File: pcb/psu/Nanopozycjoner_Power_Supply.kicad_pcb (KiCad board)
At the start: 2 copper layers, 73 x 80 mm, 132 parts, among them J1 Conn_01x02_Socket, J2 Conn_01x02_Socket, J3 Conn_01x02_Socket, J4 Conn_01x02_Socket, J5 Conn_01x02_Socket, J6 Conn_01x02_Socket, J7 Conn_01x02_Socket, J8 Conn_01x02_Socket, U1 ADPL16000B, U2 LTC3260xDE, U3 ADPL54203, U4 ADPL54203

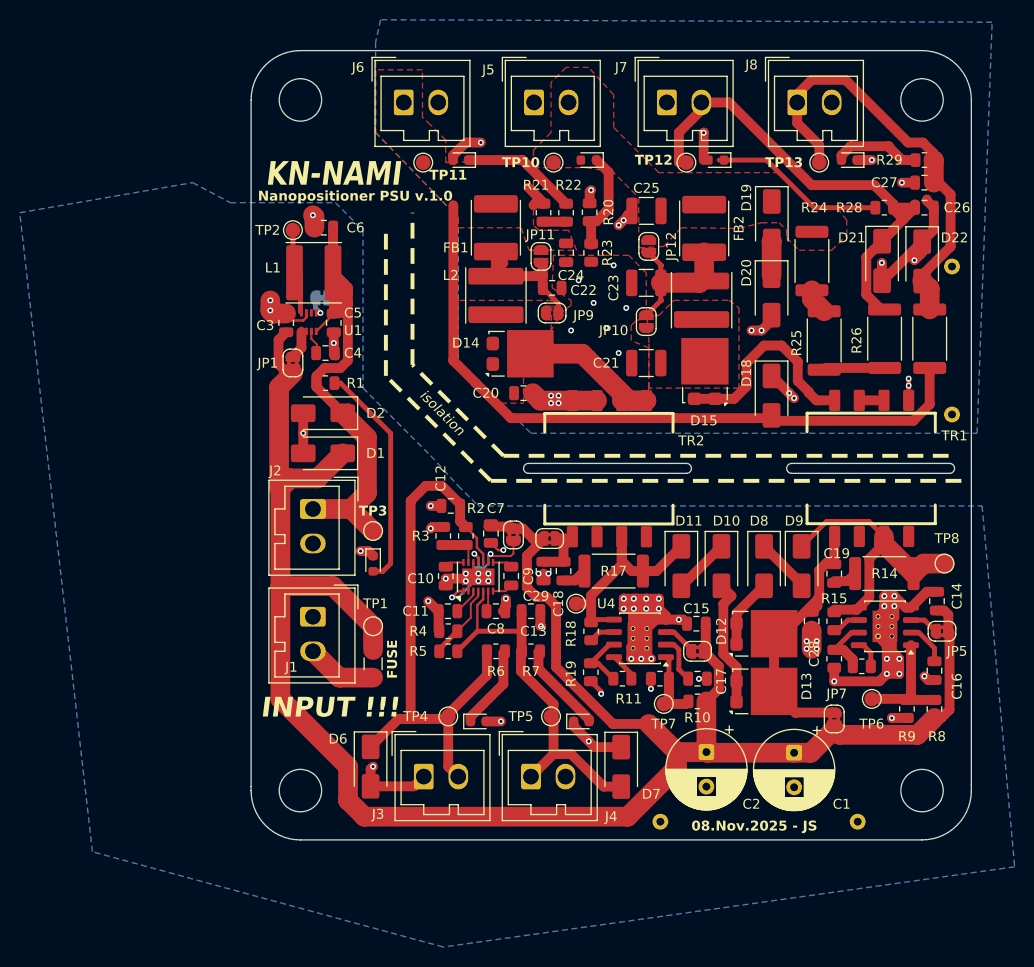
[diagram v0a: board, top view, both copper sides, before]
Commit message: final changes
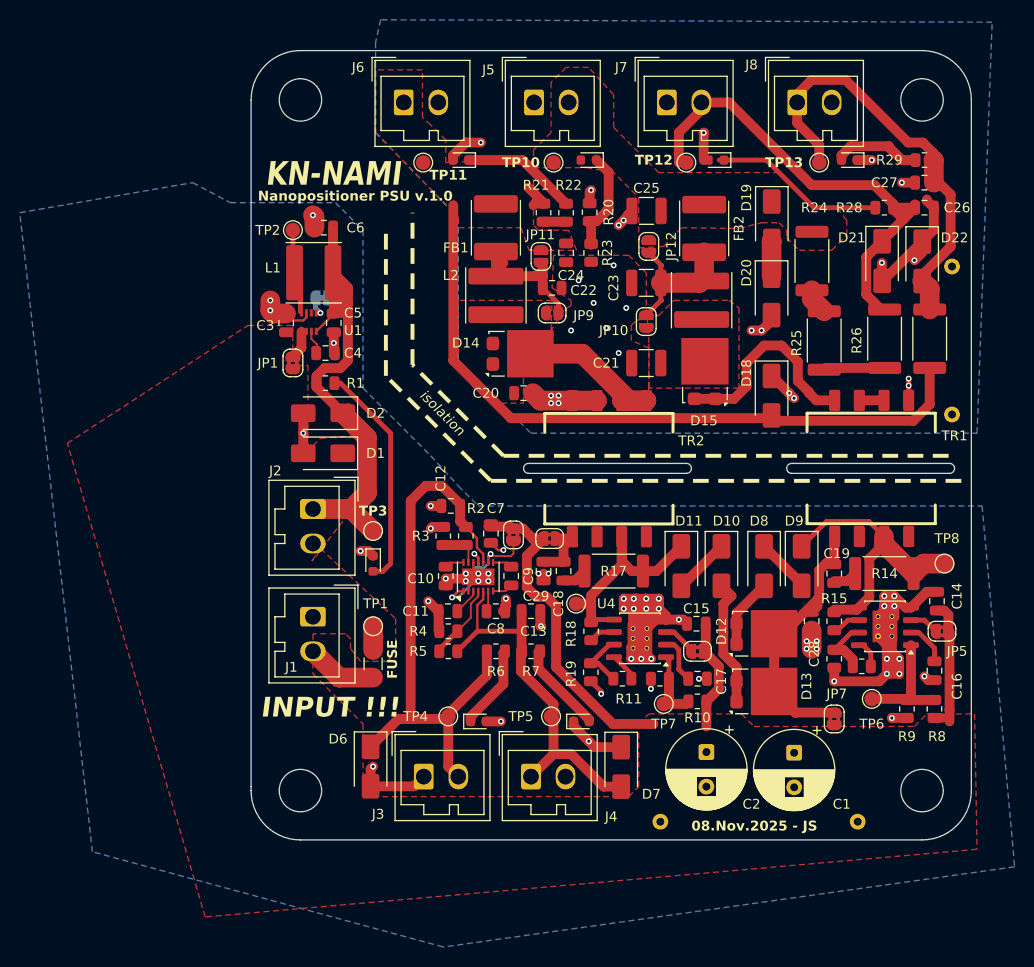
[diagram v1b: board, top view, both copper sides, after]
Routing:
- net +24V: track 206.0 -> 60.8 mm
- added copper zone on F.Cu, net +24V
